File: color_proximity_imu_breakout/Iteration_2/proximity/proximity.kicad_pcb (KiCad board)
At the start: 2 copper layers, 13 x 20 mm, 13 parts, among them IC1 VL53L4CDV0DH_1, J1 Conn_01x10, J2 Conn_01x10

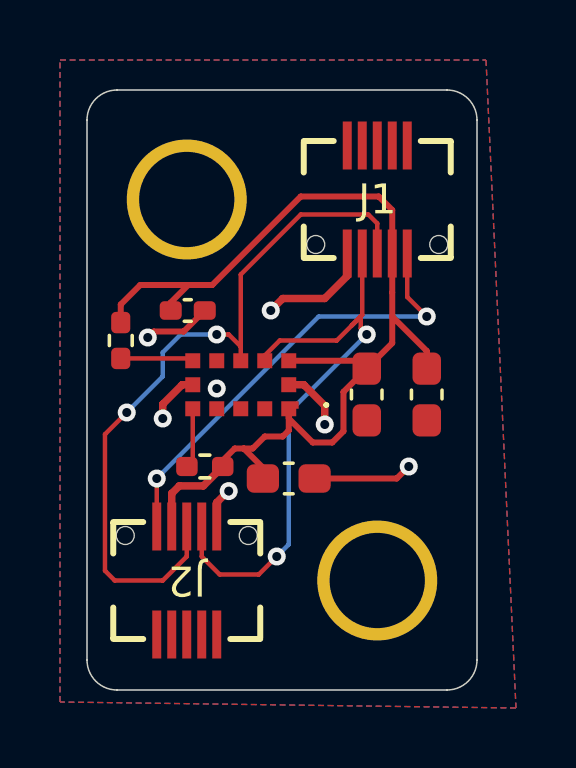
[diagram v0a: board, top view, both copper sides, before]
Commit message: updated production files
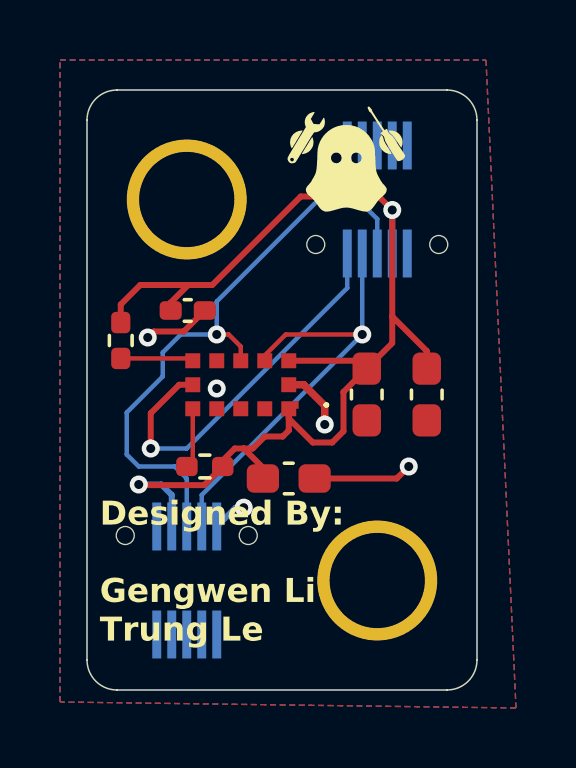
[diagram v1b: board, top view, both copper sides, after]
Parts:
- removed the G*** at (141.6, 121.5)
- added G***: LOGO, GDLX-SMT-N-66:vexu_ghost, F.Cu at (146.9, 106.8)
- J1, J2: moved to B.Cu
- moved G*** 6.64 mm to (144.7, 113.6), turned to -145 degrees
- turned C1 to -90 degrees
- turned C2 to -90 degrees
- turned J1 to 180 degrees
- turned J2 to 0 degrees
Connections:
- C1 pad 1: GND -> +3.3V
- C1 pad 2: +3.3V -> GND
- C2 pad 1: GND -> +3.3V
- C2 pad 2: +3.3V -> GND
- J1 pad 10: +5V -> GND
- J1 pad 6: GND -> unconnected-(J1-Pin_6-Pad6)
- J1 pad 7: /scl -> +3.3V
- J1 pad 9: +3.3V -> /scl
- J2 pad 10: +5V -> GND
- J2 pad 6: GND -> unconnected-(J2-Pin_6-Pad6)
- J2 pad 7: /scl -> +3.3V
- J2 pad 9: +3.3V -> /scl
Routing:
- net +5V: track 15.2 -> 0.00 mm, vias 2 -> 0
- net GND: track 14.6 -> 21.7 mm, vias 7 -> 6
- net /scl: track 19.8 -> 15.0 mm, vias 2 -> 1
- net /sda: track 24.7 -> 20.6 mm, vias 2 -> 1
- net +3.3V: track 36.8 -> 40.4 mm, vias 0 -> 2
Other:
- board text added: "Designed By: Gengwen Li Trung Le"
- board text removed: "Designed By Gengwen Li Trung Le"
